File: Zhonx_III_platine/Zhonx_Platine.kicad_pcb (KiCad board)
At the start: 2 copper layers, 35 parts, among them SW3 ON/OFF, SW4 RST, U1 MCP1700, U2 PCF8574R, U3 OLED_128X64, U4 MCMT5-F-V

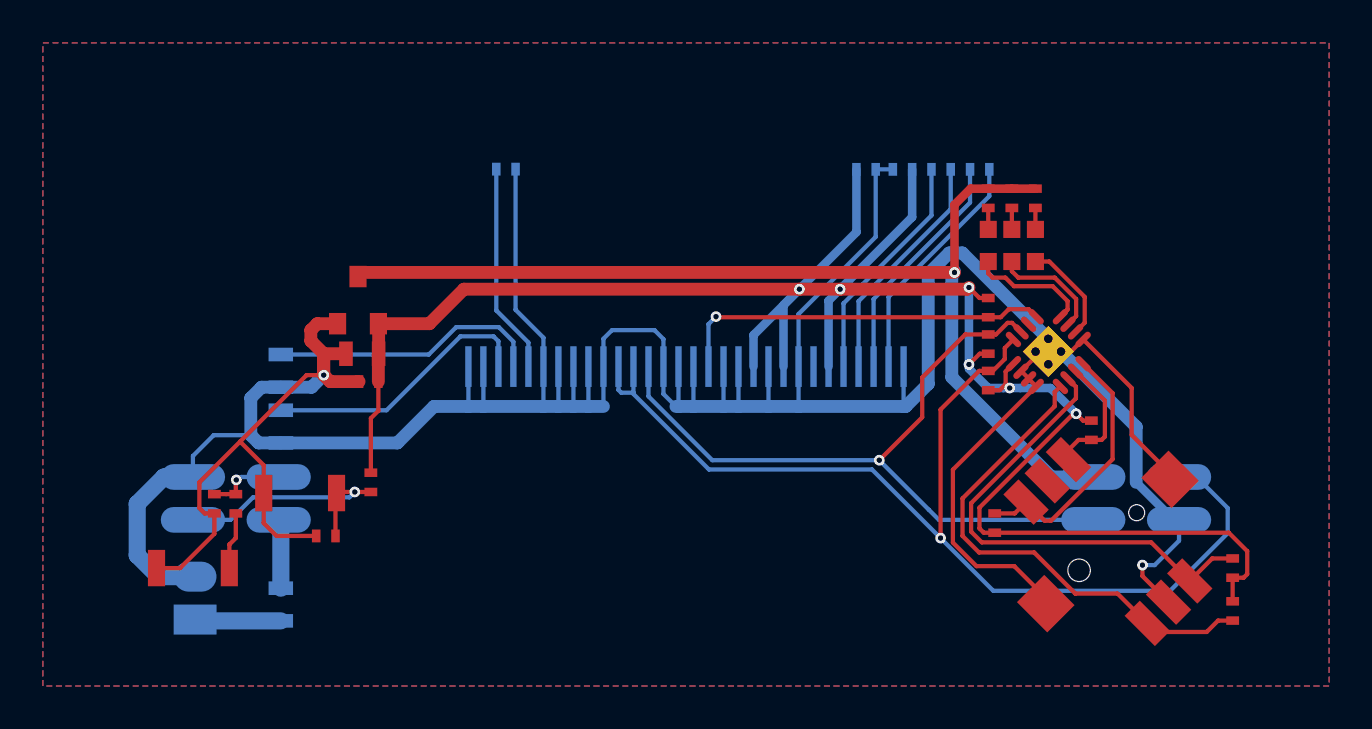
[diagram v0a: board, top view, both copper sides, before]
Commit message: Nouvelle librairie (.pretty)
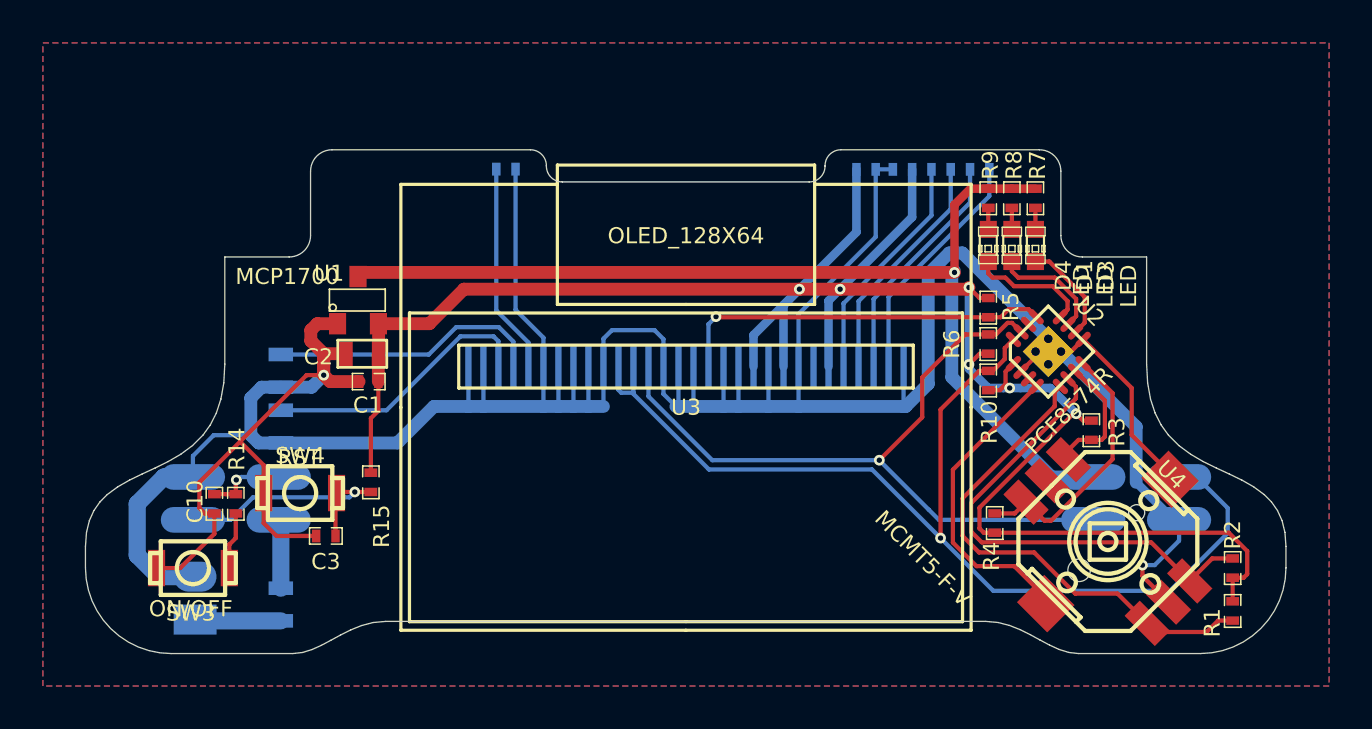
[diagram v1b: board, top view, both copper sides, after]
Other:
- board outline added: 56 x 23.5 mm
